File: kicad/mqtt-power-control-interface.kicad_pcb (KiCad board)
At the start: 2 copper layers, 16 parts, among them J1 Conn_01x04_Pin, J2 Conn_01x04_Pin, J3 Conn_01x04_Pin, J4 Conn_01x04_Pin, J5 Conn_01x04_Pin, J6 Conn_01x04_Pin, U1 LTV-847, U2 LTV-847, U3 LTV-847, U4 RPi Pico W

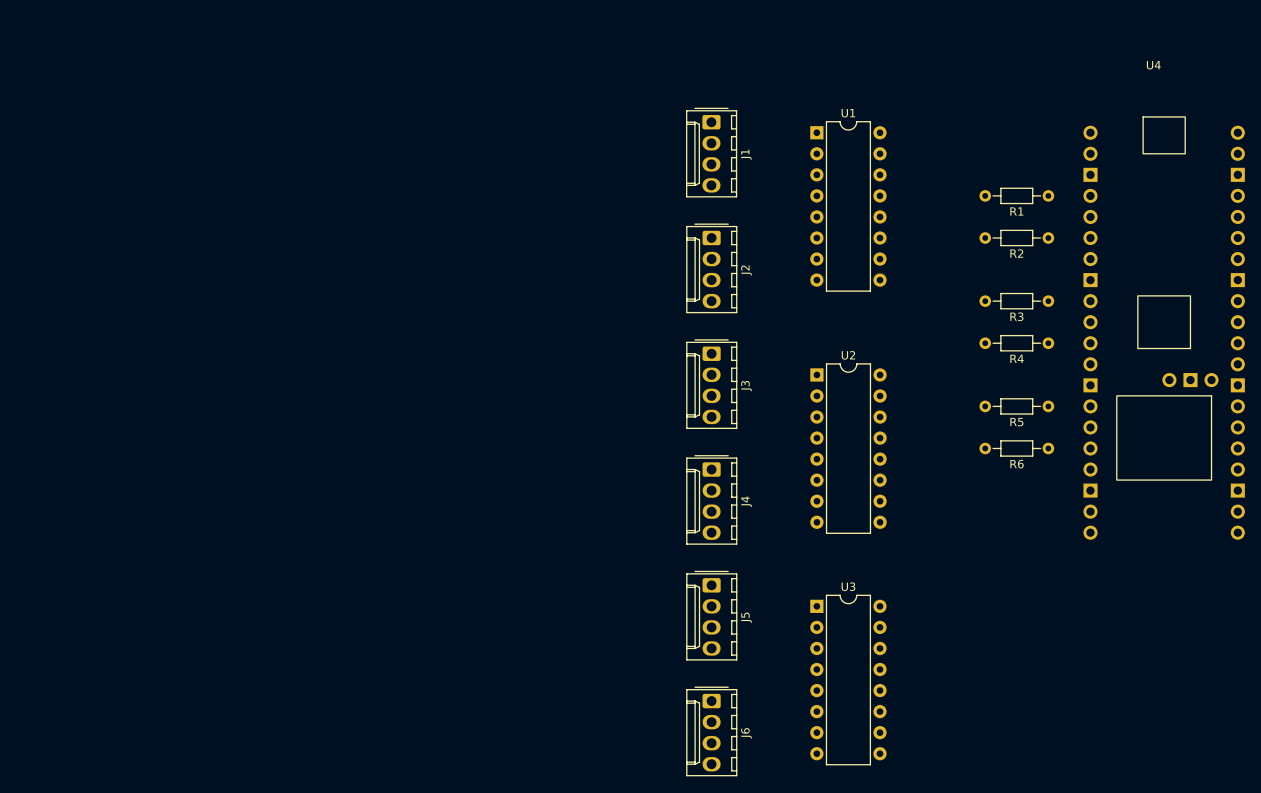
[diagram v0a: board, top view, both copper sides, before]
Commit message: Enhanced schematic and board
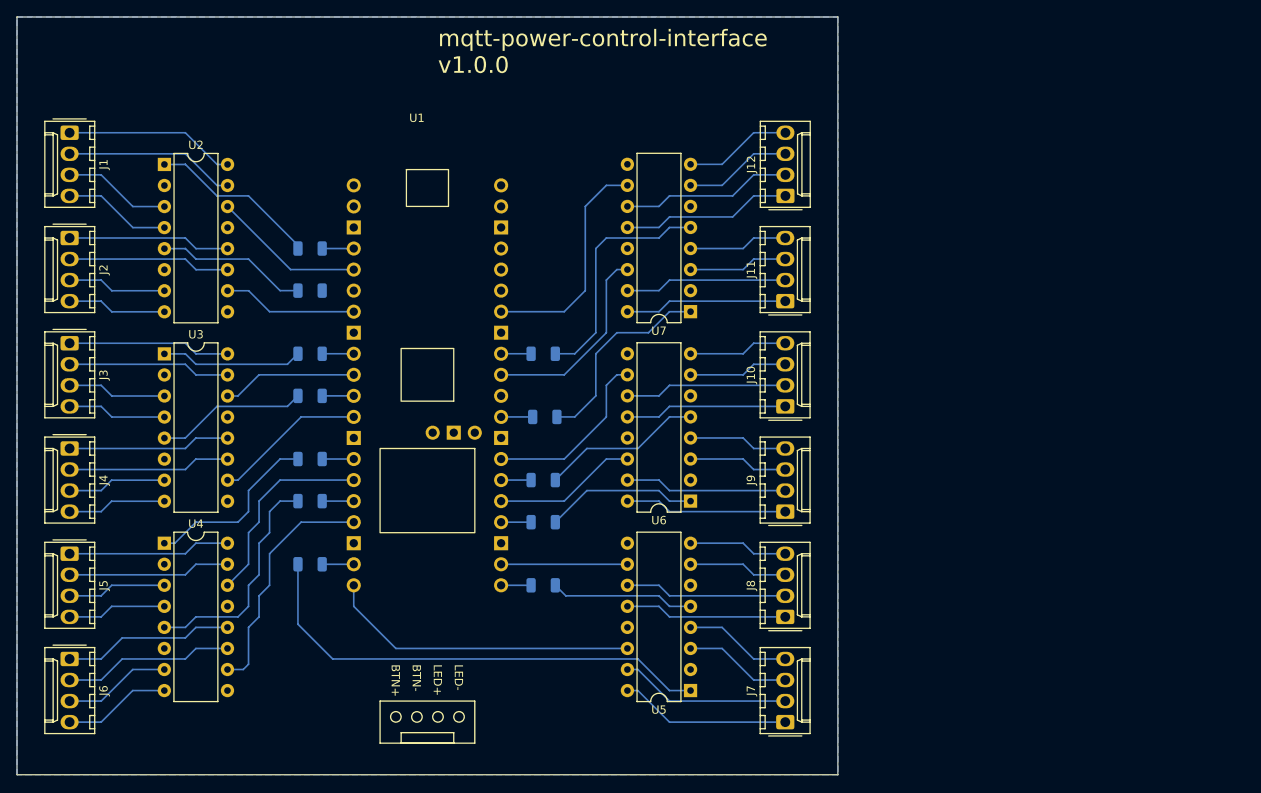
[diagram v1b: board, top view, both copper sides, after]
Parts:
- added J10: Conn_01x04_Pin, Connector_Molex:Molex_KK-254_AE-6410-04A_1x04_P2.54mm_Vertical, F.Cu at (120.7, 66.0)
- added J11: Conn_01x04_Pin, Connector_Molex:Molex_KK-254_AE-6410-04A_1x04_P2.54mm_Vertical, F.Cu at (120.7, 53.3)
- added J12: Conn_01x04_Pin, Connector_Molex:Molex_KK-254_AE-6410-04A_1x04_P2.54mm_Vertical, F.Cu at (120.7, 40.6)
- added J7: Conn_01x04_Pin, Connector_Molex:Molex_KK-254_AE-6410-04A_1x04_P2.54mm_Vertical, F.Cu at (120.7, 104.1)
- added J8: Conn_01x04_Pin, Connector_Molex:Molex_KK-254_AE-6410-04A_1x04_P2.54mm_Vertical, F.Cu at (120.7, 91.4)
- added J9: Conn_01x04_Pin, Connector_Molex:Molex_KK-254_AE-6410-04A_1x04_P2.54mm_Vertical, F.Cu at (120.7, 78.7)
- added R10: 330, Resistor_SMD:R_1206_3216Metric, B.Cu at (91.4, 74.9)
- added R11: 330, Resistor_SMD:R_1206_3216Metric, B.Cu at (91.6, 67.3)
- added R12: 330, Resistor_SMD:R_1206_3216Metric, B.Cu at (91.4, 59.7)
- added R7: 330, Resistor_SMD:R_1206_3216Metric, B.Cu at (63.3, 85.1)
- added R8: 330, Resistor_SMD:R_1206_3216Metric, B.Cu at (91.4, 87.6)
- added R9: 330, Resistor_SMD:R_1206_3216Metric, B.Cu at (91.4, 80.0)
- added U5: LTV-847, Package_DIP:DIP-16_W7.62mm, F.Cu at (109.2, 100.3)
- added U6: LTV-847, Package_DIP:DIP-16_W7.62mm, F.Cu at (109.2, 77.5)
- added U7: LTV-847, Package_DIP:DIP-16_W7.62mm, F.Cu at (109.2, 54.6)
- R1, R2, R3, R4, R5, R6: footprint Resistor_THT:R_Axial_DIN0204_L3.6mm_D1.6mm_P7.62mm_Horizontal -> Resistor_SMD:R_1206_3216Metric; moved to B.Cu
- U1: value LTV-847 -> RPi Pico W; footprint Package_DIP:DIP-16_W7.62mm -> Custom:RPI Pico W
- U4: value RPi Pico W -> LTV-847; footprint Custom:RPI Pico W -> Package_DIP:DIP-16_W7.62mm
- moved U4 132.4 mm to (45.7, 82.5)
- moved R1 89.3 mm to (63.3, 47.0)
- moved R2 89.3 mm to (63.3, 52.1)
- moved R3 89.3 mm to (63.3, 59.7)
- moved R4 89.3 mm to (63.3, 64.8)
- moved R5 89.3 mm to (63.3, 72.4)
- moved R6 89.3 mm to (63.3, 77.5)
- moved U3 84.4 mm to (45.7, 59.7)
- moved U2 82.7 mm to (45.7, 36.8)
- moved J6 77.6 mm to (34.3, 96.5)
- moved J5 77.6 mm to (34.3, 83.8)
- moved J4 77.5 mm to (34.3, 71.1)
- moved J3 77.5 mm to (34.3, 58.4)
- moved J2 77.5 mm to (34.3, 45.7)
- moved J1 77.5 mm to (34.3, 33.0)
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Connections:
- U1 pad 1: Net-(R1-Pad2) -> unconnected-(U1-GP0-Pad1)
- U1 pad 10: GPIO5 -> GPIO7
- U1 pad 11: DEV2_SW- -> GPIO8
- U1 pad 12: DEV2_SW+ -> GPIO9
- U1 pad 13: GND -> unconnected-(U1-GND3-Pad13)
- U1 pad 14: GPIO3 -> GPIO10
- U1 pad 15: DEV1_SW- -> GPIO11
- U1 pad 16: DEV1_SW+ -> GPIO12
- U1 pad 2: GND -> unconnected-(U1-GP1-Pad2)
- U1 pad 3: DEV1_LED+ -> GND
- U1 pad 4: DEV1_LED- -> GPIO2
- U1 pad 5: Net-(R2-Pad2) -> GPIO3
- U1 pad 6: GND -> GPIO4
- U1 pad 7: DEV2_LED+ -> GPIO5
- U1 pad 8: DEV2_LED- -> unconnected-(U1-GND2-Pad8)
- U1 pad 9: GND -> GPIO6
- U2 pad 1: Net-(R3-Pad2) -> Net-(R1-Pad2)
- U2 pad 10: GPIO9 -> GPIO5
- U2 pad 11: DEV4_SW- -> DEV2_SW-
- U2 pad 12: DEV4_SW+ -> DEV2_SW+
- U2 pad 14: GPIO7 -> GPIO3
- U2 pad 15: DEV3_SW- -> DEV1_SW-
- U2 pad 16: DEV3_SW+ -> DEV1_SW+
- U2 pad 3: DEV3_LED+ -> DEV1_LED+
- U2 pad 4: DEV3_LED- -> DEV1_LED-
- U2 pad 5: Net-(R4-Pad2) -> Net-(R2-Pad2)
- U2 pad 7: DEV4_LED+ -> DEV2_LED+
- U2 pad 8: DEV4_LED- -> DEV2_LED-
- U3 pad 1: Net-(R5-Pad2) -> Net-(R3-Pad2)
- U3 pad 10: GPIO13 -> GPIO9
- U3 pad 11: DEV6_SW- -> DEV4_SW-
- U3 pad 12: DEV6_SW+ -> DEV4_SW+
- U3 pad 14: GPIO11 -> GPIO7
- U3 pad 15: DEV5_SW- -> DEV3_SW-
- U3 pad 16: DEV5_SW+ -> DEV3_SW+
- U3 pad 3: DEV5_LED+ -> DEV3_LED+
- U3 pad 4: DEV5_LED- -> DEV3_LED-
- U3 pad 5: Net-(R6-Pad2) -> Net-(R4-Pad2)
- U3 pad 7: DEV6_LED+ -> DEV4_LED+
- U3 pad 8: DEV6_LED- -> DEV4_LED-
- U4 pad 1: unconnected-(U4-GP0-Pad1) -> Net-(R5-Pad2)
- U4 pad 10: GPIO7 -> GPIO13
- U4 pad 11: GPIO8 -> DEV6_SW-
- U4 pad 12: GPIO9 -> DEV6_SW+
- U4 pad 13: unconnected-(U4-GND3-Pad13) -> GND
- U4 pad 14: GPIO10 -> GPIO11
- U4 pad 15: GPIO11 -> DEV5_SW-
- U4 pad 16: GPIO12 -> DEV5_SW+
- U4 pad 2: unconnected-(U4-GP1-Pad2) -> GND
- U4 pad 3: GND -> DEV5_LED+
- U4 pad 4: GPIO2 -> DEV5_LED-
- U4 pad 5: GPIO3 -> Net-(R6-Pad2)
- U4 pad 6: GPIO4 -> GND
- U4 pad 7: GPIO5 -> DEV6_LED+
- U4 pad 8: unconnected-(U4-GND2-Pad8) -> DEV6_LED-
- U4 pad 9: GPIO6 -> GND
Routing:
- net Net-(R7-Pad2): track 0.00 -> 57.9 mm
- net GPIO15: track 0.00 -> 37.7 mm
- net GPIO13: track 0.00 -> 28.9 mm
- net Net-(R12-Pad2): track 0.00 -> 28.6 mm
- net Net-(R6-Pad2): track 0.00 -> 27.6 mm
- net GPIO28: track 0.00 -> 27.5 mm
- net Net-(R11-Pad2): track 0.00 -> 24.4 mm
- net GPIO26: track 0.00 -> 24.2 mm
- net GPIO11: track 0.00 -> 24.2 mm
- net Net-(R5-Pad2): track 0.00 -> 21.8 mm
- net GPIO21: track 0.00 -> 21.7 mm
- net DEV12_SW+: track 0.00 -> 20.6 mm
- net DEV12_SW-: track 0.00 -> 20.6 mm
- net DEV1_SW-: track 0.00 -> 20.6 mm
- net DEV1_SW+: track 0.00 -> 20.6 mm
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- added copper zone on B.Cu, net GND
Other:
- board outline added: 99.1 x 91.4 mm
- rule pad_to_mask_clearance: 0 -> 0.038
- board text added: "BTN+"
- board text added: "BTN-"
- board text added: "JLCJLCJLCJLC"
- board text added: "LED+"
- board text added: "LED-"
- board text added: "mqtt-power-control-interface v1.0.0"
